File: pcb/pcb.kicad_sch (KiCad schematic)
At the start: 22 parts, among them J1 LED 1 5V/GND/DIN/DOUT, J2 LED 2 5V/GND/DIN/DOUT, J3 LED 3 5V/GND/DIN/DOUT, J4 LED 4 5V/GND/DIN/DOUT, J5 LED 5 5V/GND/DIN/DOUT, J6 LED 6 5V/GND/DIN/DOUT, J7 LED 7 5V/GND/DIN/DOUT, J8 LED 8 5V/GND/DIN/DOUT, U1 ESP32-C3-SUPER-MINI, U2 74AHCT125

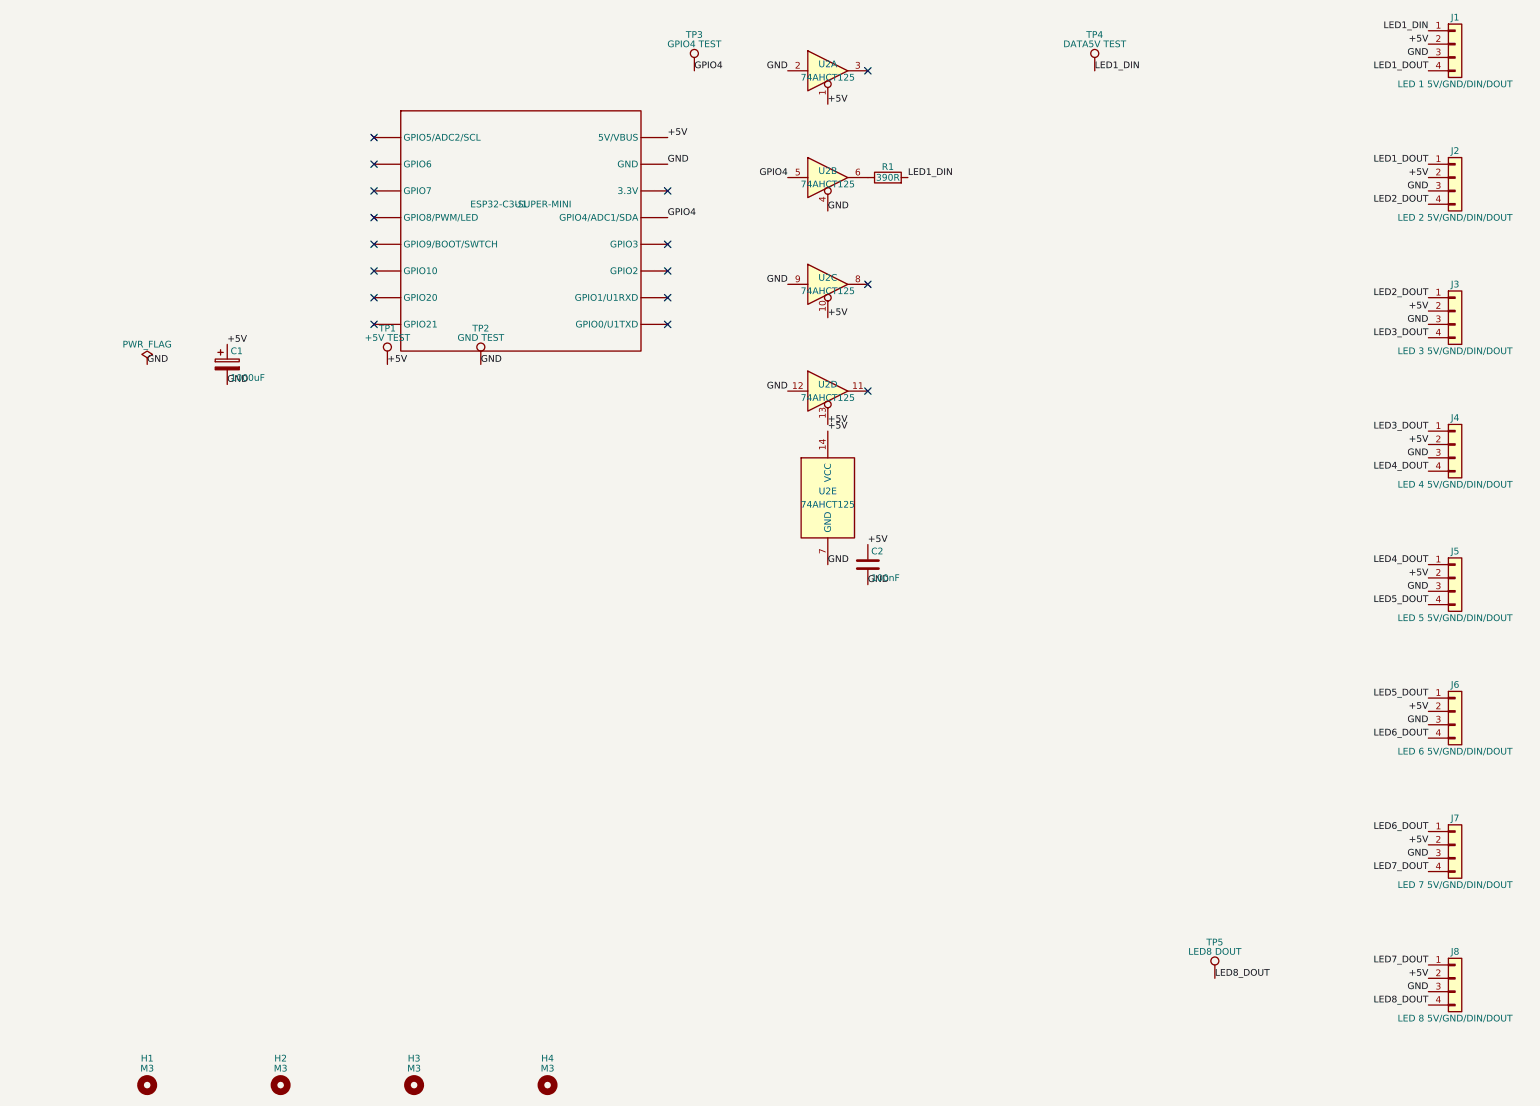
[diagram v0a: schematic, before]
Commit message: update pcb files
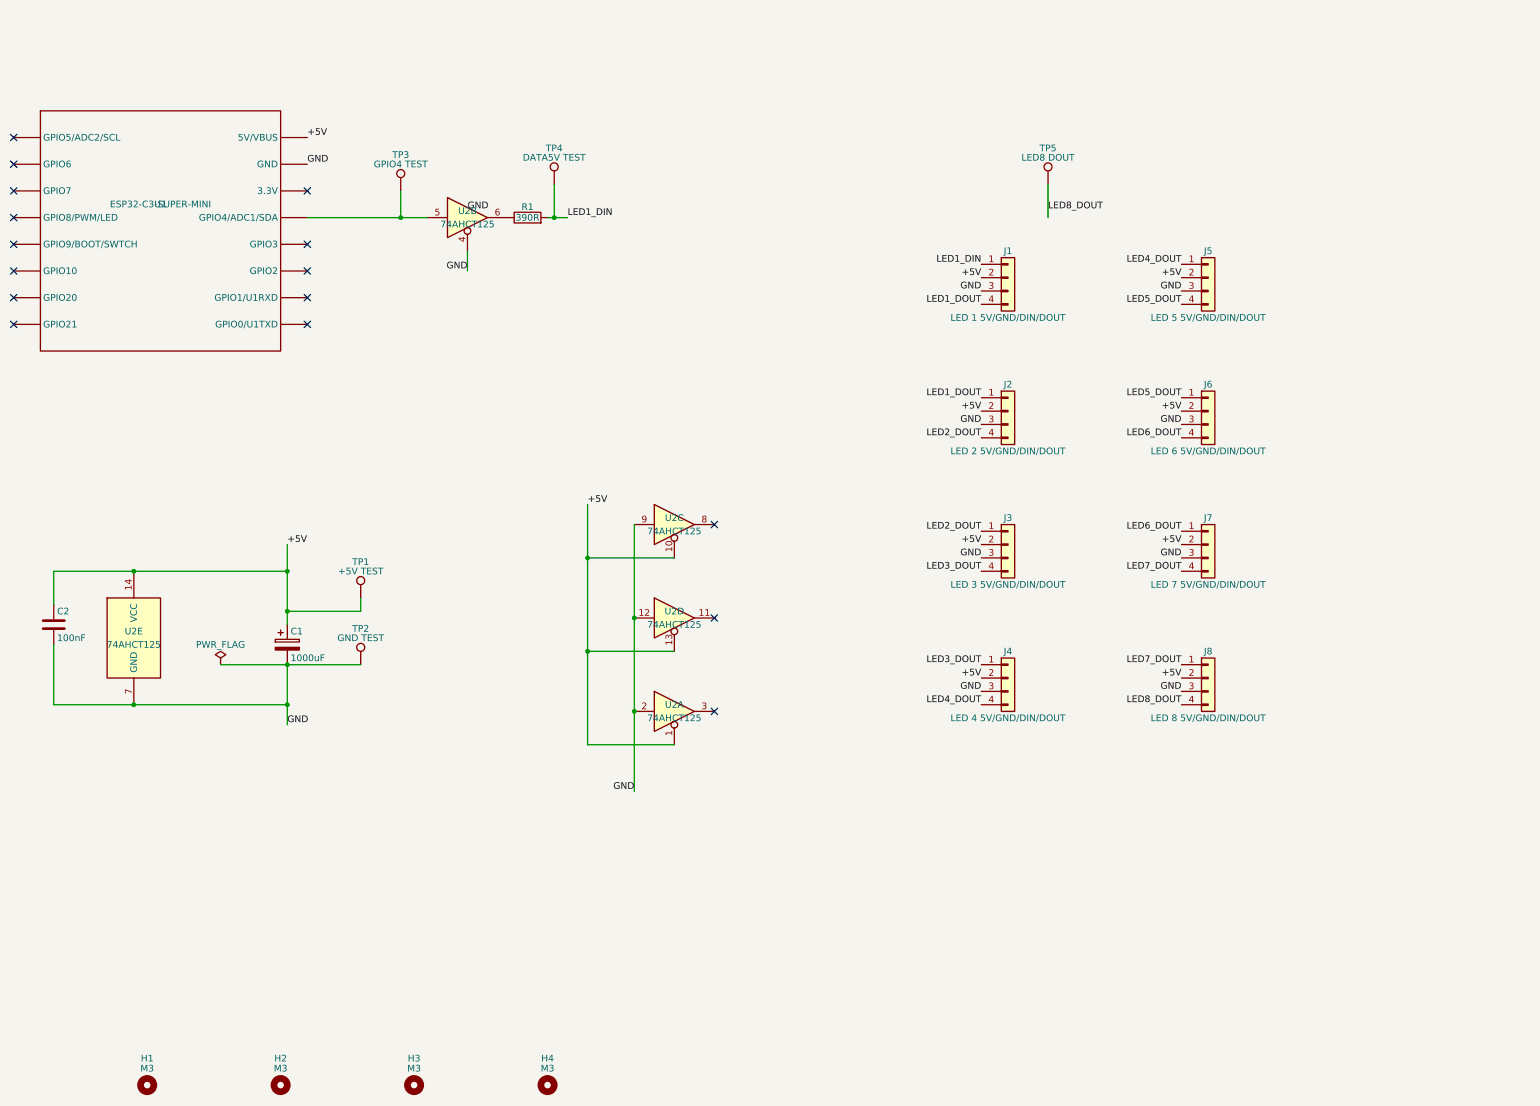
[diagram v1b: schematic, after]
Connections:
- net GPIO4: no longer names the net of TP3.1, U1.13 (GPIO4/ADC1/SDA), U2.5
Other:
- title: (none) -> Factorio Lamp ESP32-C3 board
- moved on the sheet: C1, C2, J1, J2, J3, J4, J5, J6, J7, J8, R1, TP1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
